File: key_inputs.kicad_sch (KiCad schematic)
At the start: 48 parts, among them IC1 CD4051BE, IC2 CD4051BE, IC3 CD4051BE, IC4 CD4051BE, IC5 CD4051BE, IC6 CD4051BE, J1 Conn_01x06, J10 Conn_01x06, J6 Conn_01x06, J7 Conn_01x06, J8 Conn_01x06, J9 Conn_01x06

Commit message: layout and routing finished
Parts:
- R1, R10, R11, R12, R13, R14, R15, R16, R17, R18, R19, R2, R20, R21, R22, R23, R24, R25, R26, R27, R28, R29, R3, R30, R35, R36, R37, R38, R39, R4, R40, R5, R6, R7, R8, R9: footprint Resistor_THT:R_Axial_DIN0204_L3.6mm_D1.6mm_P5.08mm_Vertical -> Resistor_THT:R_Axial_DIN0204_L3.6mm_D1.6mm_P5.08mm_Horizontal
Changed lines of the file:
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@@
 			)
 		)
-		(property "Footprint" "Resistor_THT:R_Axial_DIN0204_L3.6mm_D1.6mm_P5.08mm_Vertical"
+		(property "Footprint" "Resistor_THT:R_Axial_DIN0204_L3.6mm_D1.6mm_P5.08mm_Horizontal"
 			(at 70.612 181.61 90)
 			(effects
@@
 			)
 		)
-		(property "Footprint" "Resistor_THT:R_Axial_DIN0204_L3.6mm_D1.6mm_P5.08mm_Vertical"
+		(property "Footprint" "Resistor_THT:R_Axial_DIN0204_L3.6mm_D1.6mm_P5.08mm_Horizontal"
 			(at 87.122 99.06 90)
 			(effects
@@
 			)
 		)
-		(property "Footprint" "Resistor_THT:R_Axial_DIN0204_L3.6mm_D1.6mm_P5.08mm_Vertical"
+		(property "Footprint" "Resistor_THT:R_Axial_DIN0204_L3.6mm_D1.6mm_P5.08mm_Horizontal"
 			(at 78.232 184.15 90)
 			(effects
@@
 			)
 		)
-		(property "Footprint" "Resistor_THT:R_Axial_DIN0204_L3.6mm_D1.6mm_P5.08mm_Vertical"
+		(property "Footprint" "Resistor_THT:R_Axial_DIN0204_L3.6mm_D1.6mm_P5.08mm_Horizontal"
 			(at 62.992 120.65 90)
 			(effects
@@
 			)
 		)
-		(property "Footprint" "Resistor_THT:R_Axial_DIN0204_L3.6mm_D1.6mm_P5.08mm_Vertical"
+		(property "Footprint" "Resistor_THT:R_Axial_DIN0204_L3.6mm_D1.6mm_P5.08mm_Horizontal"
 			(at 70.612 93.98 90)
 			(effects
@@
 			)
 		)
-		(property "Footprint" "Resistor_THT:R_Axial_DIN0204_L3.6mm_D1.6mm_P5.08mm_Vertical"
+		(property "Footprint" "Resistor_THT:R_Axial_DIN0204_L3.6mm_D1.6mm_P5.08mm_Horizontal"
 			(at 55.372 176.53 90)
 			(effects
@@
 			)
 		)
-		(property "Footprint" "Resistor_THT:R_Axial_DIN0204_L3.6mm_D1.6mm_P5.08mm_Vertical"
+		(property "Footprint" "Resistor_THT:R_Axial_DIN0204_L3.6mm_D1.6mm_P5.08mm_Horizontal"
 			(at 47.752 144.78 90)
 			(effects
@@
 			)
 		)
-		(property "Footprint" "Resistor_THT:R_Axial_DIN0204_L3.6mm_D1.6mm_P5.08mm_Vertical"
+		(property "Footprint" "Resistor_THT:R_Axial_DIN0204_L3.6mm_D1.6mm_P5.08mm_Horizontal"
 			(at 55.372 147.32 90)
 			(effects
@@
 			)
 		)
-		(property "Footprint" "Resistor_THT:R_Axial_DIN0204_L3.6mm_D1.6mm_P5.08mm_Vertical"
+		(property "Footprint" "Resistor_THT:R_Axial_DIN0204_L3.6mm_D1.6mm_P5.08mm_Horizontal"
 			(at 70.612 152.4 90)
 			(effects
@@
 			)
 		)
-		(property "Footprint" "Resistor_THT:R_Axial_DIN0204_L3.6mm_D1.6mm_P5.08mm_Vertical"
+		(property "Footprint" "Resistor_THT:R_Axial_DIN0204_L3.6mm_D1.6mm_P5.08mm_Horizontal"
 			(at 47.752 173.99 90)
 			(effects
@@
 			)
 		)
-		(property "Footprint" "Resistor_THT:R_Axial_DIN0204_L3.6mm_D1.6mm_P5.08mm_Vertical"
+		(property "Footprint" "Resistor_THT:R_Axial_DIN0204_L3.6mm_D1.6mm_P5.08mm_Horizontal"
 			(at 80.772 67.31 90)
 			(effects
@@
 			)
 		)
-		(property "Footprint" "Resistor_THT:R_Axial_DIN0204_L3.6mm_D1.6mm_P5.08mm_Vertical"
+		(property "Footprint" "Resistor_THT:R_Axial_DIN0204_L3.6mm_D1.6mm_P5.08mm_Horizontal"
 			(at 73.152 64.77 90)
 			(effects
@@
 			)
 		)
-		(property "Footprint" "Resistor_THT:R_Axial_DIN0204_L3.6mm_D1.6mm_P5.08mm_Vertical"
+		(property "Footprint" "Resistor_THT:R_Axial_DIN0204_L3.6mm_D1.6mm_P5.08mm_Horizontal"
 			(at 87.122 186.69 90)
 			(effects
@@
 			)
 		)
-		(property "Footprint" "Resistor_THT:R_Axial_DIN0204_L3.6mm_D1.6mm_P5.08mm_Vertical"
+		(property "Footprint" "Resistor_THT:R_Axial_DIN0204_L3.6mm_D1.6mm_P5.08mm_Horizontal"
 			(at 70.612 123.19 90)
 			(effects
@@
 			)
 		)
-		(property "Footprint" "Resistor_THT:R_Axial_DIN0204_L3.6mm_D1.6mm_P5.08mm_Vertical"
+		(property "Footprint" "Resistor_THT:R_Axial_DIN0204_L3.6mm_D1.6mm_P5.08mm_Horizontal"
 			(at 78.232 125.73 90)
 			(effects
@@
 			)
 		)
-		(property "Footprint" "Resistor_THT:R_Axial_DIN0204_L3.6mm_D1.6mm_P5.08mm_Vertical"
+		(property "Footprint" "Resistor_THT:R_Axial_DIN0204_L3.6mm_D1.6mm_P5.08mm_Horizontal"
 			(at 62.992 149.86 90)
 			(effects
@@
 			)
 		)
-		(property "Footprint" "Resistor_THT:R_Axial_DIN0204_L3.6mm_D1.6mm_P5.08mm_Vertical"
+		(property "Footprint" "Resistor_THT:R_Axial_DIN0204_L3.6mm_D1.6mm_P5.08mm_Horizontal"
 			(at 50.292 27.94 90)
 			(effects
@@
 			)
 		)
-		(property "Footprint" "Resistor_THT:R_Axial_DIN0204_L3.6mm_D1.6mm_P5.08mm_Vertical"
+		(property "Footprint" "Resistor_THT:R_Axial_DIN0204_L3.6mm_D1.6mm_P5.08mm_Horizontal"
 			(at 89.662 40.64 90)
 			(effects
@@
 			)
 		)
-		(property "Footprint" "Resistor_THT:R_Axial_DIN0204_L3.6mm_D1.6mm_P5.08mm_Vertical"
+		(property "Footprint" "Resistor_THT:R_Axial_DIN0204_L3.6mm_D1.6mm_P5.08mm_Horizontal"
 			(at 87.122 157.48 90)
 			(effects
@@
 			)
 		)
-		(property "Footprint" "Resistor_THT:R_Axial_DIN0204_L3.6mm_D1.6mm_P5.08mm_Vertical"
+		(property "Footprint" "Resistor_THT:R_Axial_DIN0204_L3.6mm_D1.6mm_P5.08mm_Horizontal"
 			(at 55.372 118.11 90)
 			(effects
@@
 			)
 		)
-		(property "Footprint" "Resistor_THT:R_Axial_DIN0204_L3.6mm_D1.6mm_P5.08mm_Vertical"
+		(property "Footprint" "Resistor_THT:R_Axial_DIN0204_L3.6mm_D1.6mm_P5.08mm_Horizontal"
 			(at 50.292 57.15 90)
 			(effects
@@
 			)
 		)
-		(property "Footprint" "Resistor_THT:R_Axial_DIN0204_L3.6mm_D1.6mm_P5.08mm_Vertical"
+		(property "Footprint" "Resistor_THT:R_Axial_DIN0204_L3.6mm_D1.6mm_P5.08mm_Horizontal"
 			(at 57.912 59.69 90)
 			(effects
@@
 			)
 		)
-		(property "Footprint" "Resistor_THT:R_Axial_DIN0204_L3.6mm_D1.6mm_P5.08mm_Vertical"
+		(property "Footprint" "Resistor_THT:R_Axial_DIN0204_L3.6mm_D1.6mm_P5.08mm_Horizontal"
 			(at 78.232 96.52 90)
 			(effects
@@
 			)
 		)
-		(property "Footprint" "Resistor_THT:R_Axial_DIN0204_L3.6mm_D1.6mm_P5.08mm_Vertical"
+		(property "Footprint" "Resistor_THT:R_Axial_DIN0204_L3.6mm_D1.6mm_P5.08mm_Horizontal"
 			(at 62.992 91.44 90)
 			(effects
@@
 			)
 		)
-		(property "Footprint" "Resistor_THT:R_Axial_DIN0204_L3.6mm_D1.6mm_P5.08mm_Vertical"
+		(property "Footprint" "Resistor_THT:R_Axial_DIN0204_L3.6mm_D1.6mm_P5.08mm_Horizontal"
 			(at 62.992 179.07 90)
 			(effects
@@
 			)
 		)
-		(property "Footprint" "Resistor_THT:R_Axial_DIN0204_L3.6mm_D1.6mm_P5.08mm_Vertical"
+		(property "Footprint" "Resistor_THT:R_Axial_DIN0204_L3.6mm_D1.6mm_P5.08mm_Horizontal"
 			(at 87.122 128.27 90)
 			(effects
@@
 			)
 		)
-		(property "Footprint" "Resistor_THT:R_Axial_DIN0204_L3.6mm_D1.6mm_P5.08mm_Vertical"
+		(property "Footprint" "Resistor_THT:R_Axial_DIN0204_L3.6mm_D1.6mm_P5.08mm_Horizontal"
 			(at 89.662 69.85 90)
 			(effects
@@
 			)
 		)
-		(property "Footprint" "Resistor_THT:R_Axial_DIN0204_L3.6mm_D1.6mm_P5.08mm_Vertical"
+		(property "Footprint" "Resistor_THT:R_Axial_DIN0204_L3.6mm_D1.6mm_P5.08mm_Horizontal"
 			(at 57.912 30.48 90)
 			(effects
@@
 			)
 		)
-		(property "Footprint" "Resistor_THT:R_Axial_DIN0204_L3.6mm_D1.6mm_P5.08mm_Vertical"
+		(property "Footprint" "Resistor_THT:R_Axial_DIN0204_L3.6mm_D1.6mm_P5.08mm_Horizontal"
 			(at 55.372 88.9 90)
 			(effects
@@
 			)
 		)
-		(property "Footprint" "Resistor_THT:R_Axial_DIN0204_L3.6mm_D1.6mm_P5.08mm_Vertical"
+		(property "Footprint" "Resistor_THT:R_Axial_DIN0204_L3.6mm_D1.6mm_P5.08mm_Horizontal"
 			(at 47.752 86.36 90)
 			(effects
@@
 			)
 		)
-		(property "Footprint" "Resistor_THT:R_Axial_DIN0204_L3.6mm_D1.6mm_P5.08mm_Vertical"
+		(property "Footprint" "Resistor_THT:R_Axial_DIN0204_L3.6mm_D1.6mm_P5.08mm_Horizontal"
 			(at 65.532 33.02 90)
 			(effects
@@
 			)
 		)
-		(property "Footprint" "Resistor_THT:R_Axial_DIN0204_L3.6mm_D1.6mm_P5.08mm_Vertical"
+		(property "Footprint" "Resistor_THT:R_Axial_DIN0204_L3.6mm_D1.6mm_P5.08mm_Horizontal"
 			(at 80.772 38.1 90)
 			(effects
@@
 			)
 		)
-		(property "Footprint" "Resistor_THT:R_Axial_DIN0204_L3.6mm_D1.6mm_P5.08mm_Vertical"
+		(property "Footprint" "Resistor_THT:R_Axial_DIN0204_L3.6mm_D1.6mm_P5.08mm_Horizontal"
 			(at 73.152 35.56 90)
 			(effects
@@
 			)
 		)
-		(property "Footprint" "Resistor_THT:R_Axial_DIN0204_L3.6mm_D1.6mm_P5.08mm_Vertical"
+		(property "Footprint" "Resistor_THT:R_Axial_DIN0204_L3.6mm_D1.6mm_P5.08mm_Horizontal"
 			(at 65.532 62.23 90)
 			(effects
@@
 			)
 		)
-		(property "Footprint" "Resistor_THT:R_Axial_DIN0204_L3.6mm_D1.6mm_P5.08mm_Vertical"
+		(property "Footprint" "Resistor_THT:R_Axial_DIN0204_L3.6mm_D1.6mm_P5.08mm_Horizontal"
 			(at 78.232 154.94 90)
 			(effects
@@
 			)
 		)
-		(property "Footprint" "Resistor_THT:R_Axial_DIN0204_L3.6mm_D1.6mm_P5.08mm_Vertical"
+		(property "Footprint" "Resistor_THT:R_Axial_DIN0204_L3.6mm_D1.6mm_P5.08mm_Horizontal"
 			(at 47.752 115.57 90)
 			(effects

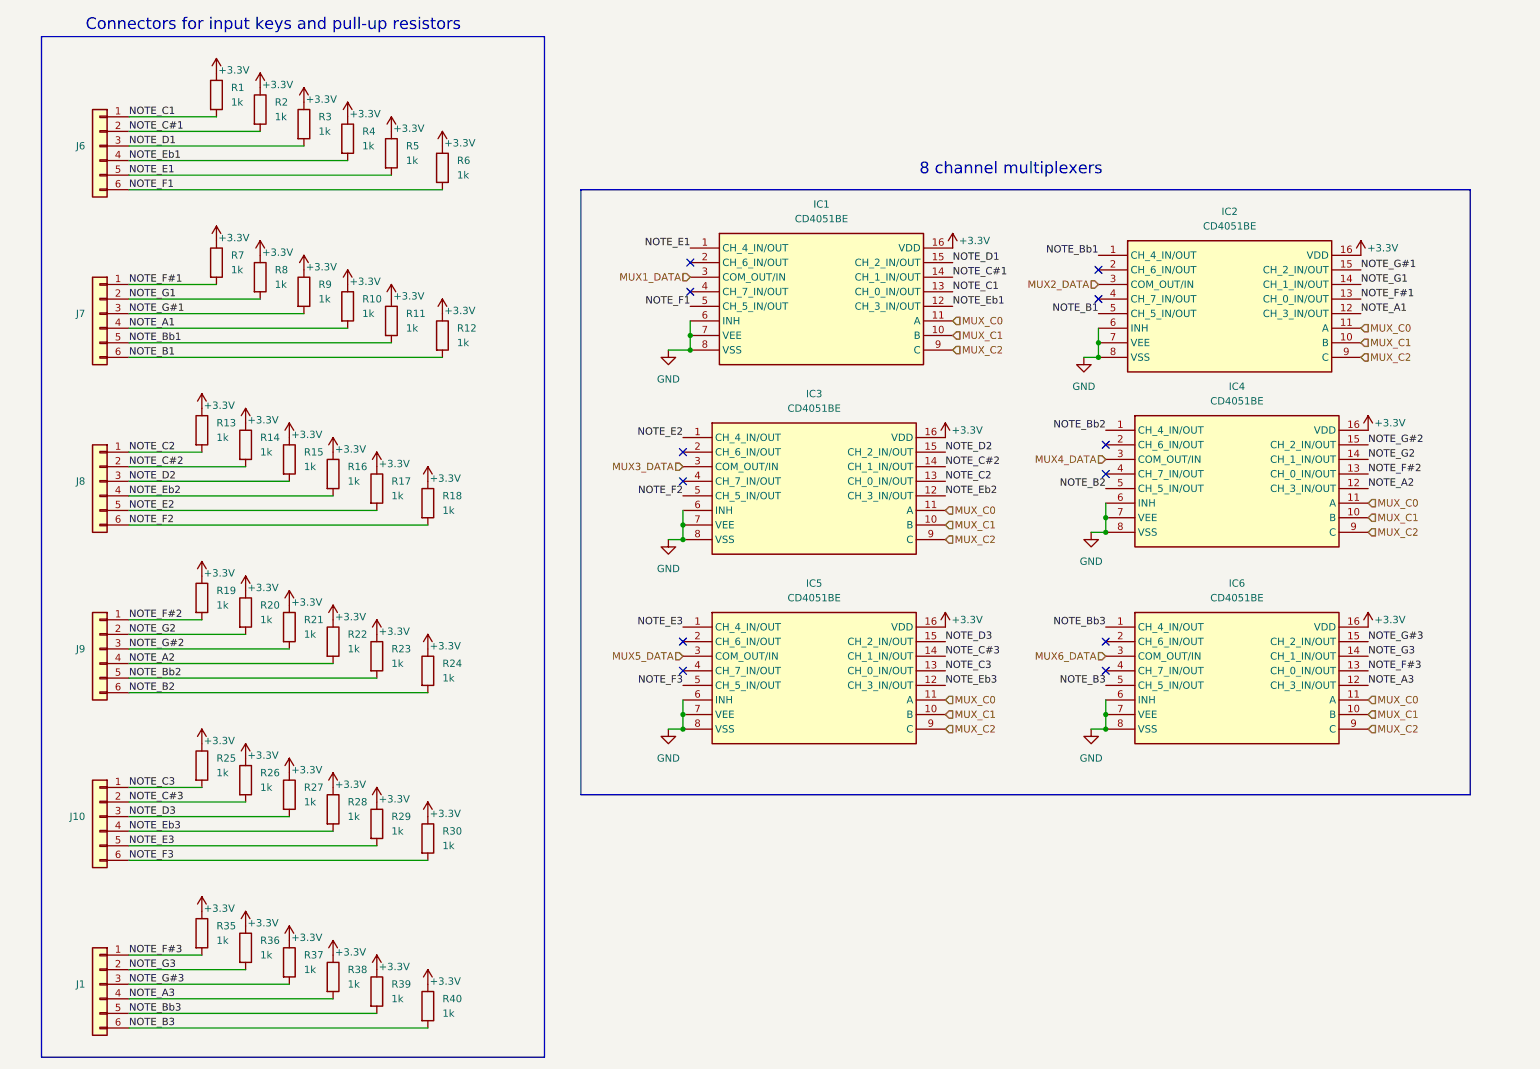
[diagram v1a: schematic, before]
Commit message: BREAKING: production
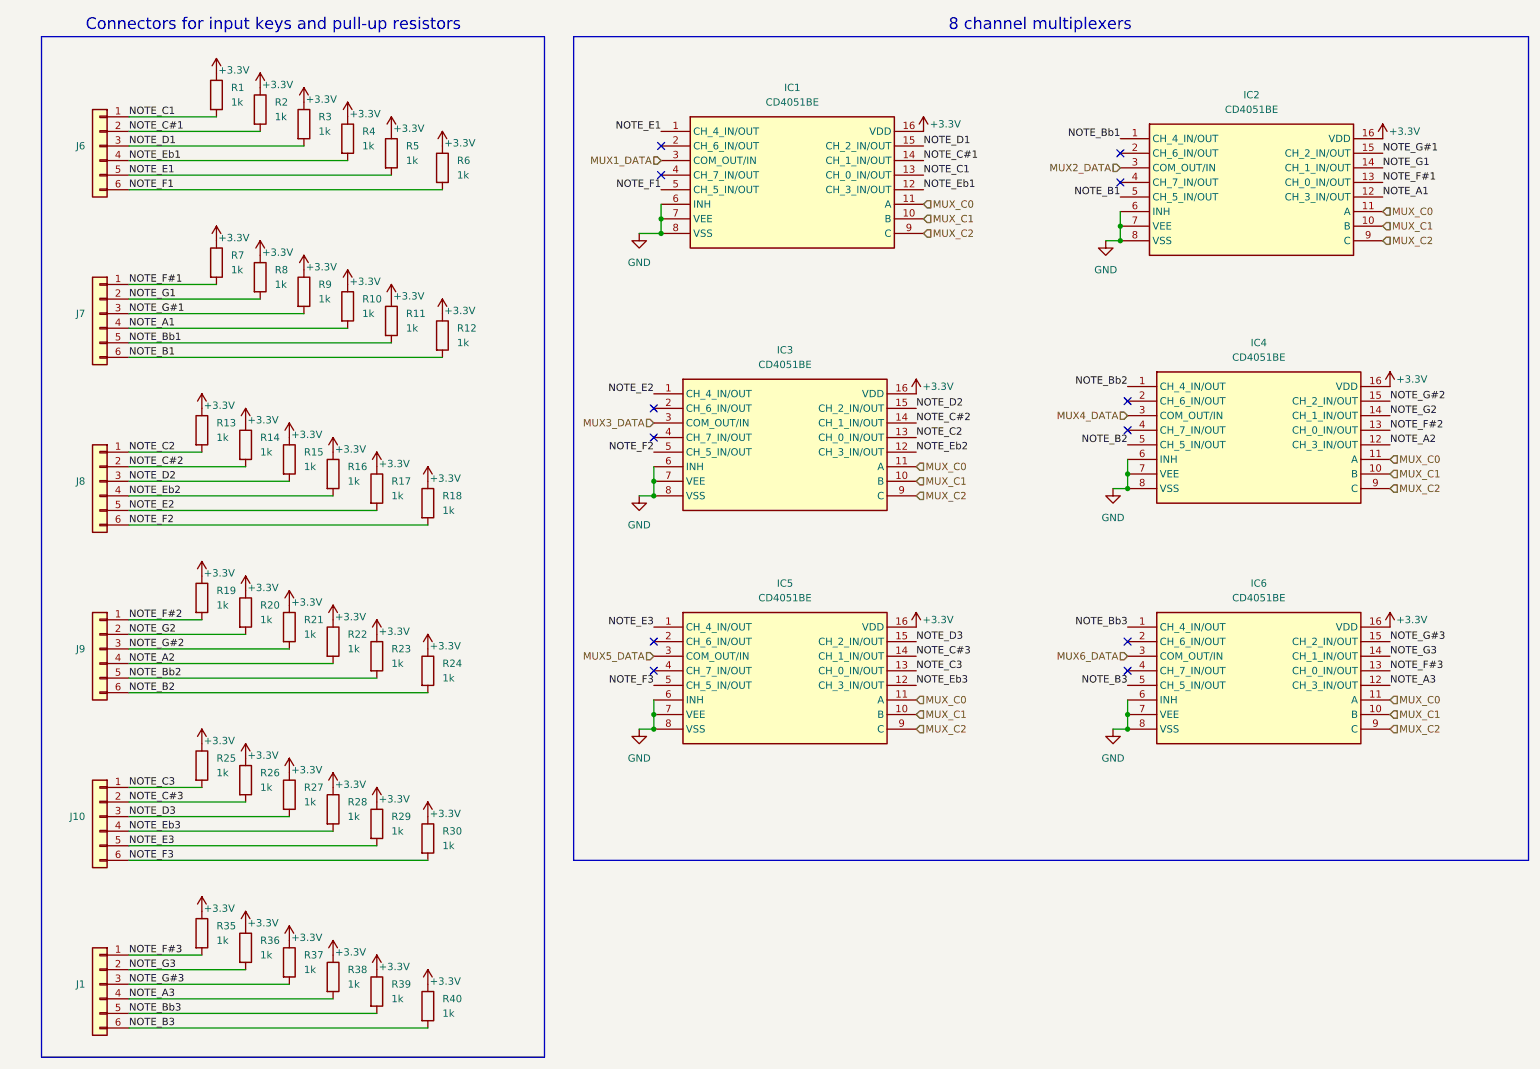
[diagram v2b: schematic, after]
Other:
- moved on the sheet: IC1, IC2, IC3, IC4, IC5, IC6
